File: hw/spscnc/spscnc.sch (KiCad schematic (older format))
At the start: 7 parts

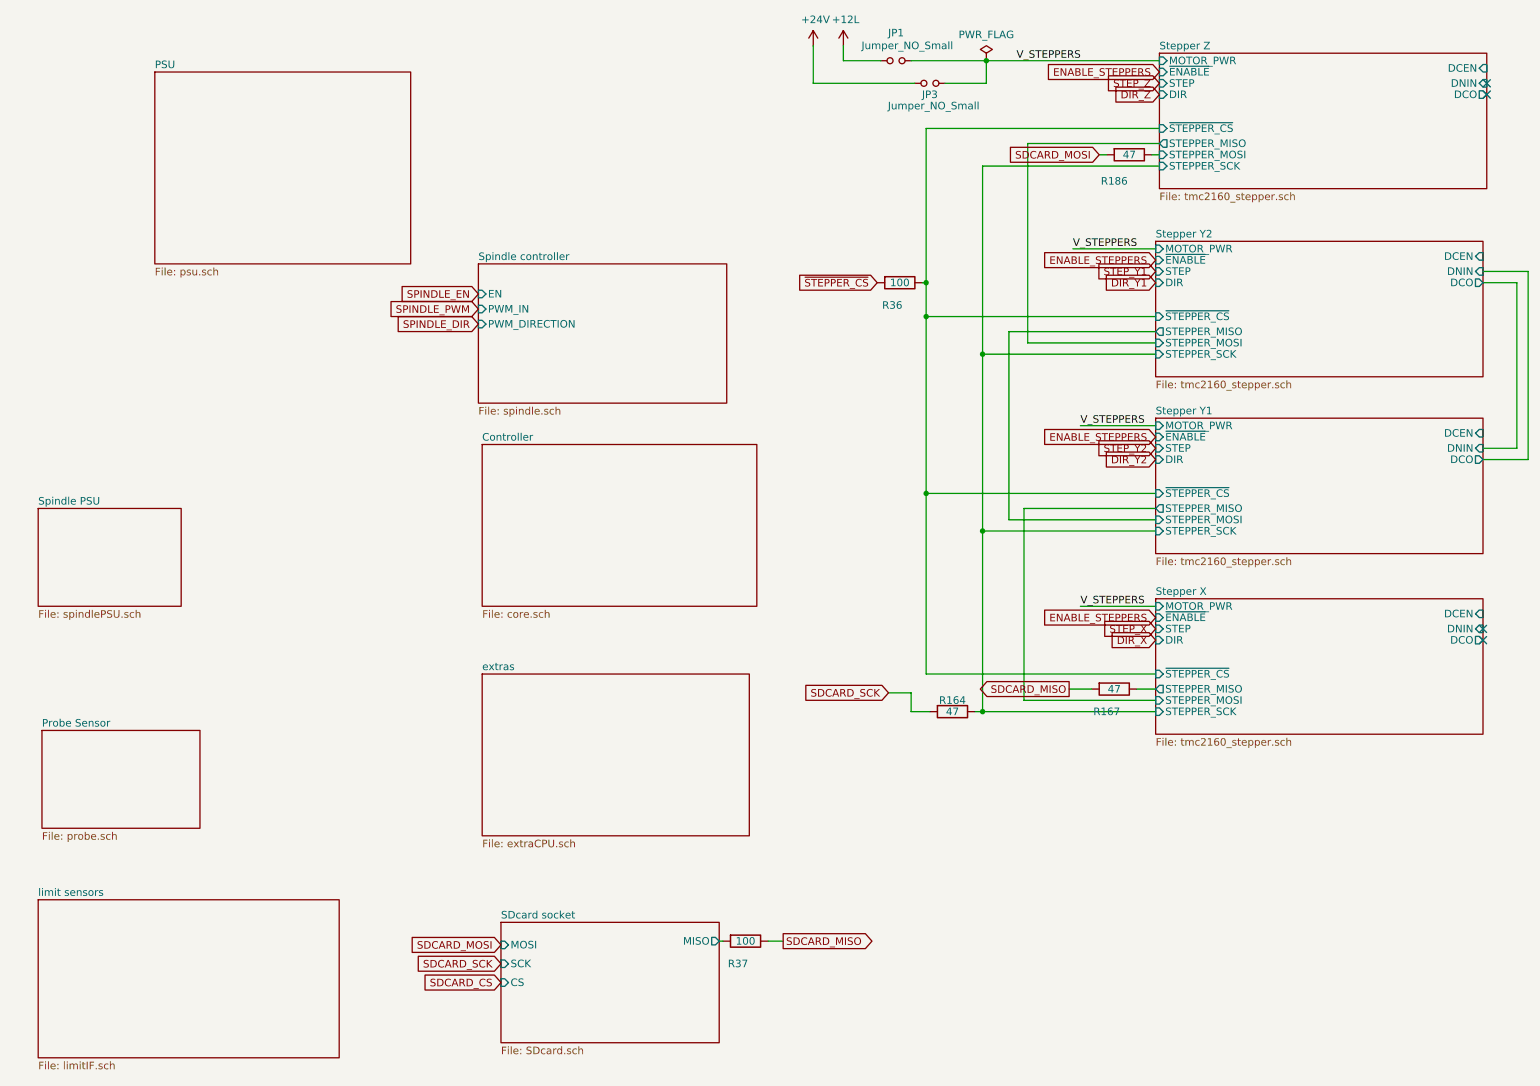
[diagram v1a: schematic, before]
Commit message: halfway changes to support additional axis and to extend over i2so
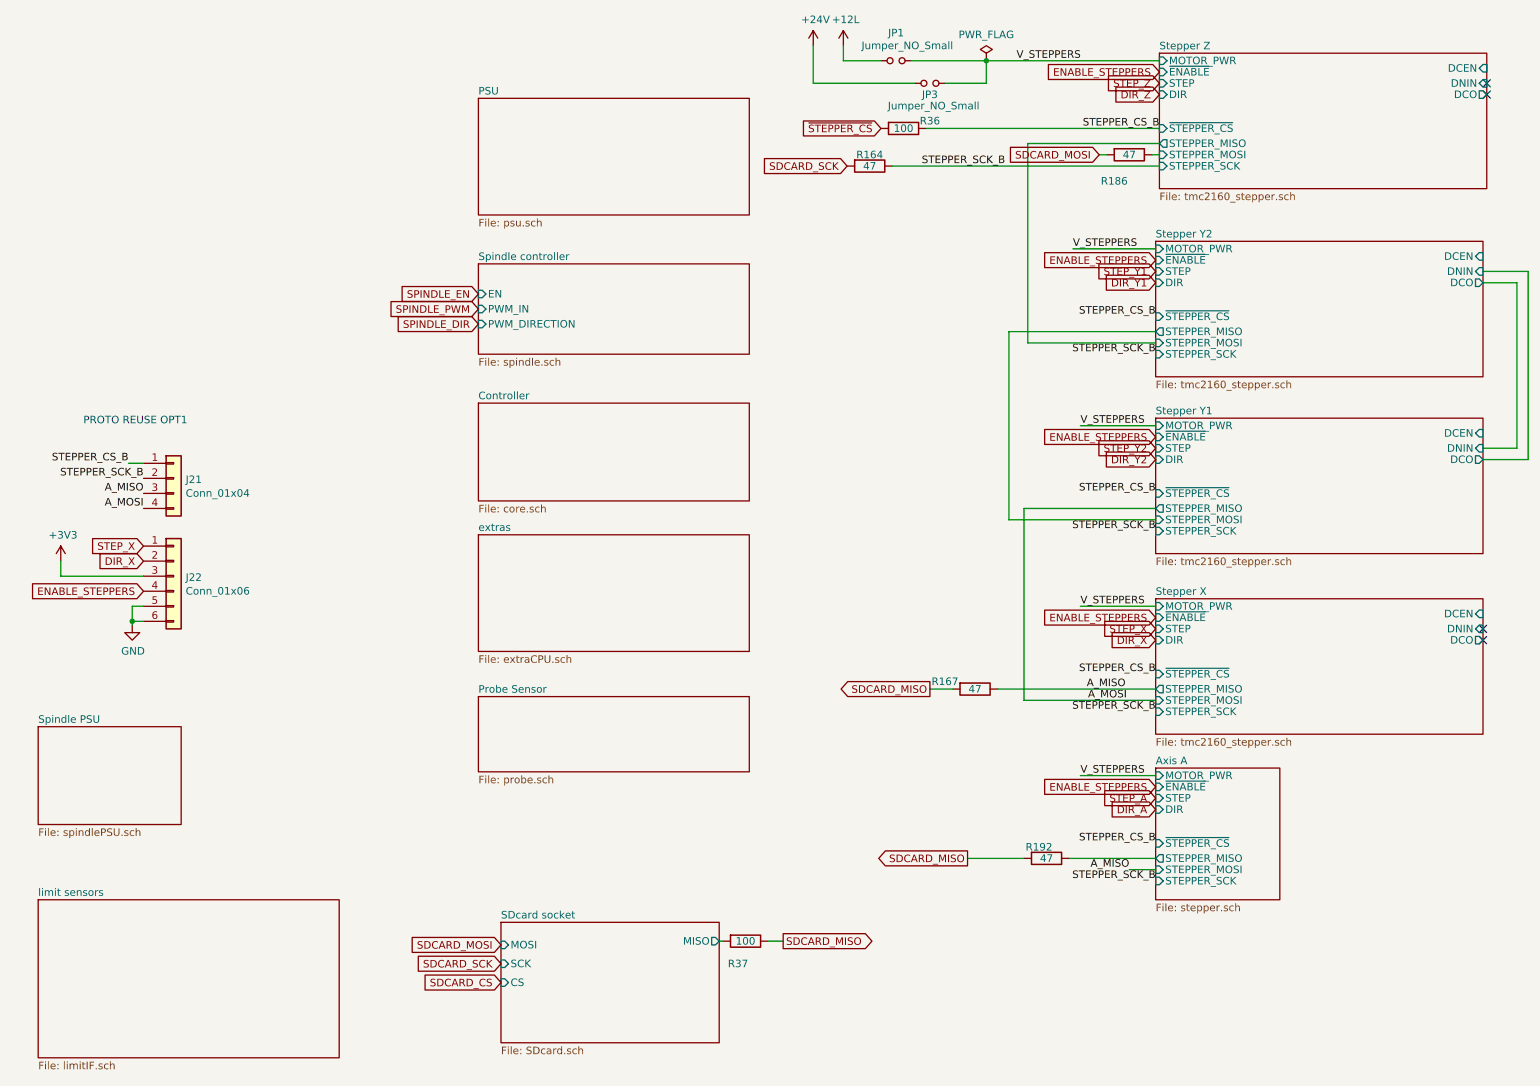
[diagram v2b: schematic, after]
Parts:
- added J21: Conn_01x04, Connector_PinHeader_2.54mm:PinHeader_1x04_P2.54mm_Vertical, symbol Connector_Generic:Conn_01x04
- added J22: Conn_01x06, Connector_PinHeader_2.54mm:PinHeader_1x06_P2.54mm_Vertical, symbol Connector_Generic:Conn_01x06
- added R192: 47, Resistor_SMD:R_0805_2012Metric, symbol Device:R
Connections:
- net DIR_X: now also J22.2 (Pin_2)
- net ENABLE_STEPPERS: now also J22.4 (Pin_4)
- net SDCARD_MISO: now also R192.2
- net STEP_X: now also J22.1 (Pin_1)
- net Stepper X/STEPPER_MISO renamed A_MISO
- net A_MISO: now also J21.3 (Pin_3)
- net Stepper X/STEPPER_SCK renamed STEPPER_SCK_B
- net STEPPER_SCK_B: now also J21.2 (Pin_2)
- net Stepper X/~STEPPER_CS renamed STEPPER_CS_B
- net STEPPER_CS_B: now also J21.1 (Pin_1)
- new net +3V3: J22.3 (Pin_3)
- new net A_MOSI: J21.4 (Pin_4)
- new net Axis A/STEPPER_MISO: R192.1
- new net GND: J22.5 (Pin_5), J22.6 (Pin_6)
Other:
- note added: "PROTO REUSE OPT1\n"
- moved on the sheet: R164, R167, R36
